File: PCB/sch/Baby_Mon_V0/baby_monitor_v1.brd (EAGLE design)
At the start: 20 x 20 mm, 44 parts, among them J1 BATT-COIN1CR1216, U1 NRF5340-QKAA-AB0-R, U2 MAX30101EFD+, U5 MAX32664GTGA+, X1 XRCGB32M000F2P10R0, Y1 CRYSTAL_OSCILLATOR0.126X0.061

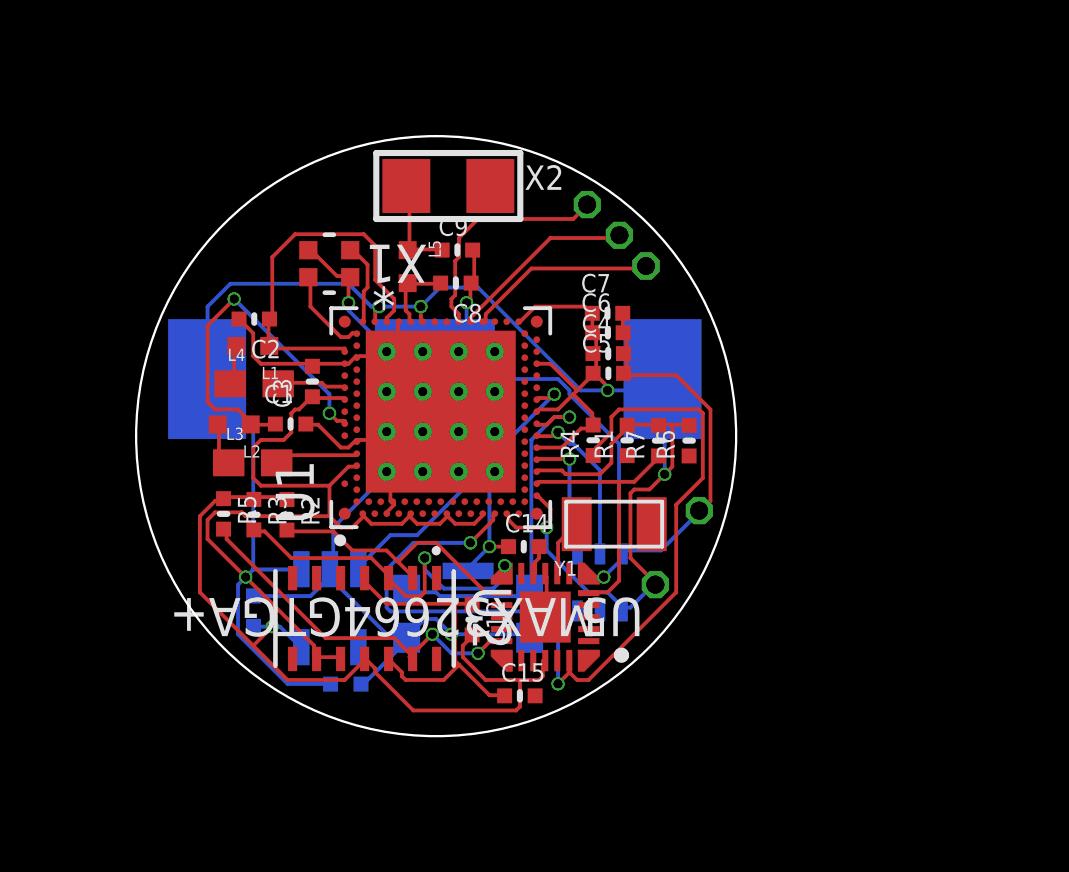
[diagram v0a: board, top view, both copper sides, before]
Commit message: u
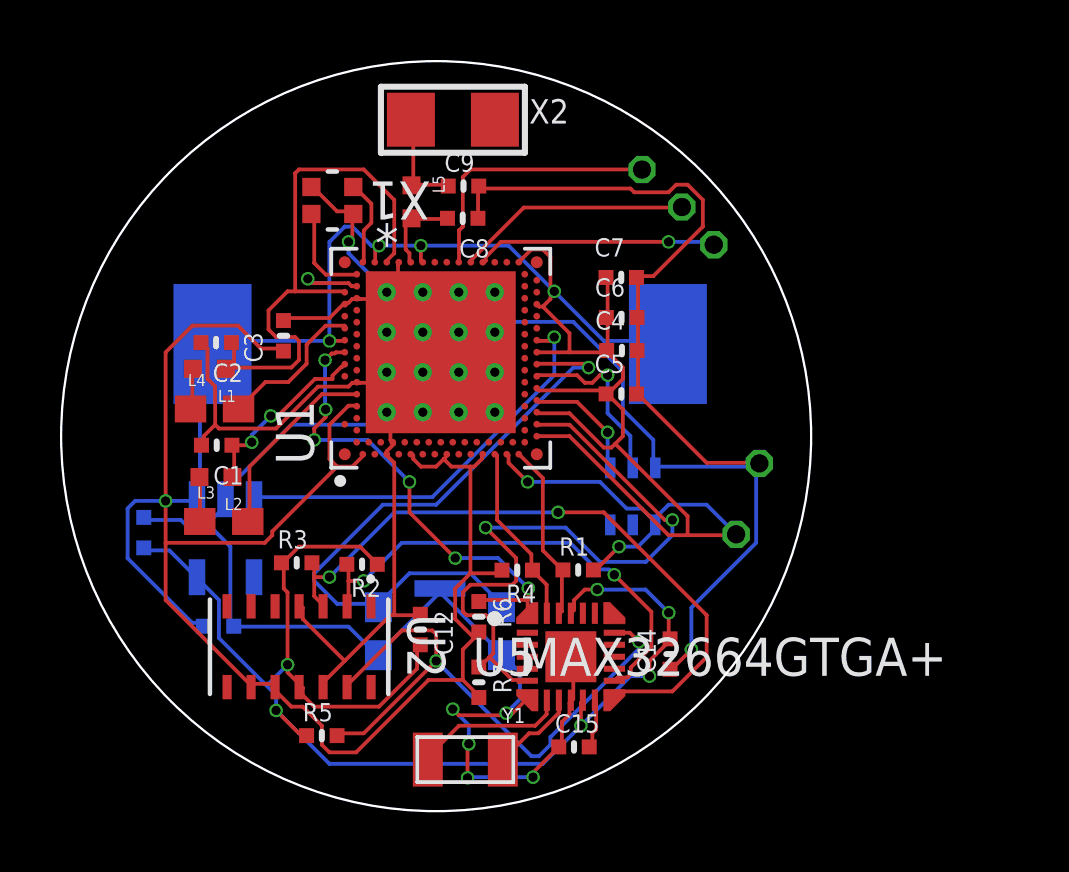
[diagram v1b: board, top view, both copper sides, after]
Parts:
- moved R7 10.0 mm to (7.26, 1.19), turned to 270 degrees
- moved Y1 9.29 mm to (6.81, -1.38), turned to 180 degrees
- moved R6 9.14 mm to (7.26, 3.38), turned to 270 degrees
- moved R5 8.09 mm to (2.03, -0.58), turned to 0 degrees
- moved C14 6.05 mm to (13.6, 2.13), turned to 90 degrees
- moved R4 5.02 mm to (8.54, 4.93), turned to 180 degrees
- moved C10 4.66 mm to (-1.41, 3.06)
- moved R1 4.62 mm to (10.6, 4.94), turned to 0 degrees
- moved C11 4.50 mm to (-3.90, 6.18)
- moved U4 4.19 mm to (-1.18, 6.00)
- moved J8 3.17 mm to (15.8, 6.12)
- moved U$2 3.07 mm to (12.4, 7.39)
- moved R2 3.00 mm to (3.37, 5.13), turned to 180 degrees
- moved C1 2.56 mm to (-1.47, 9.10), turned to 180 degrees
- moved J7 2.55 mm to (16.6, 8.49)
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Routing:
- net GND: track 112.0 -> 146.6 mm, vias 5 -> 7
- net 3.3V: track 101.7 -> 132.6 mm, vias 6 -> 8
- net SCL: track 30.5 -> 6.04 mm, vias 2 -> 0
- net 1.8V: track 28.0 -> 45.7 mm, vias 1 -> 6
- net MFIO: track 0.00 -> 16.1 mm, vias 0 -> 6
- net RST: track 8.93 -> 22.6 mm, vias 0 -> 2
- net SEN_SDA: track 12.4 -> 22.0 mm
- net SW: track 12.1 -> 21.7 mm
- net HR_INT: track 12.2 -> 20.0 mm
- net SEN_SCL: track 9.33 -> 16.0 mm, vias 0 -> 2
- net N$8: track 12.5 -> 18.9 mm
- net N$9: track 12.2 -> 6.19 mm
- net SDA: track 0.00 -> 5.98 mm
- net N$15: track 0.00 -> 5.10 mm
- net 1_8V_EN: track 9.78 -> 13.6 mm
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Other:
- board size 20 x 20 mm -> 25 x 25 mm
